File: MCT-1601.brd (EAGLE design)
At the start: 26.7 x 23.8 mm, 14 parts, among them J1 DUT, J2 Button, J3 D I/O, J5 A In, J6 Pwr, Q1 BC327

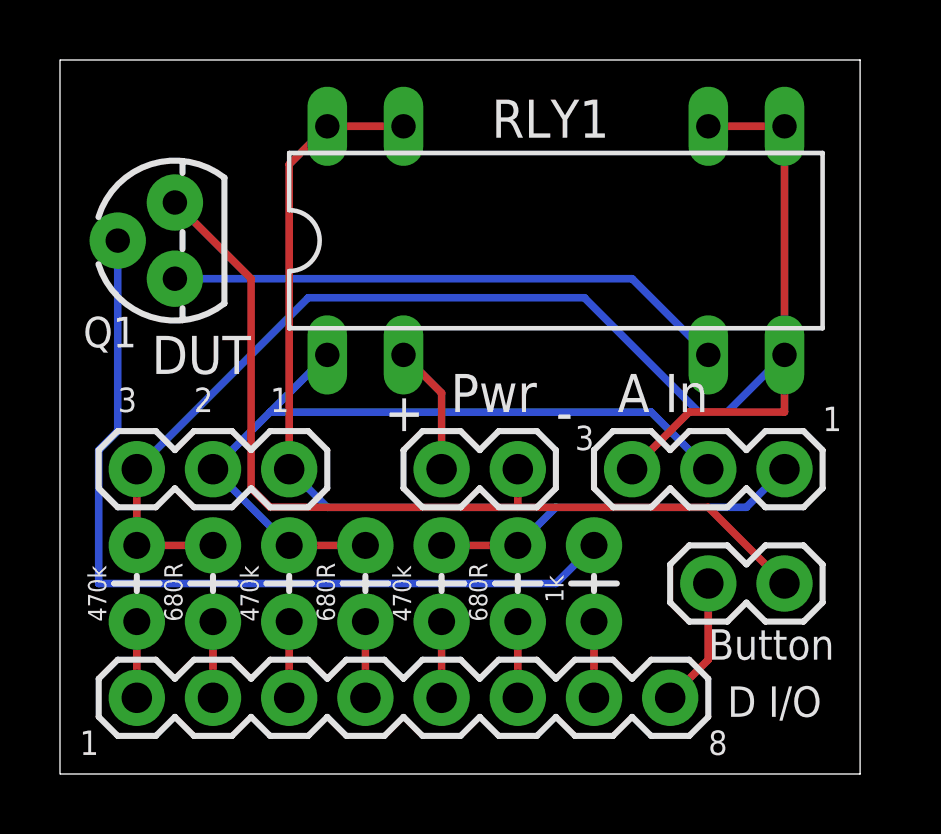
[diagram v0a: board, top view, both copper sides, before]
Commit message: Add files via upload
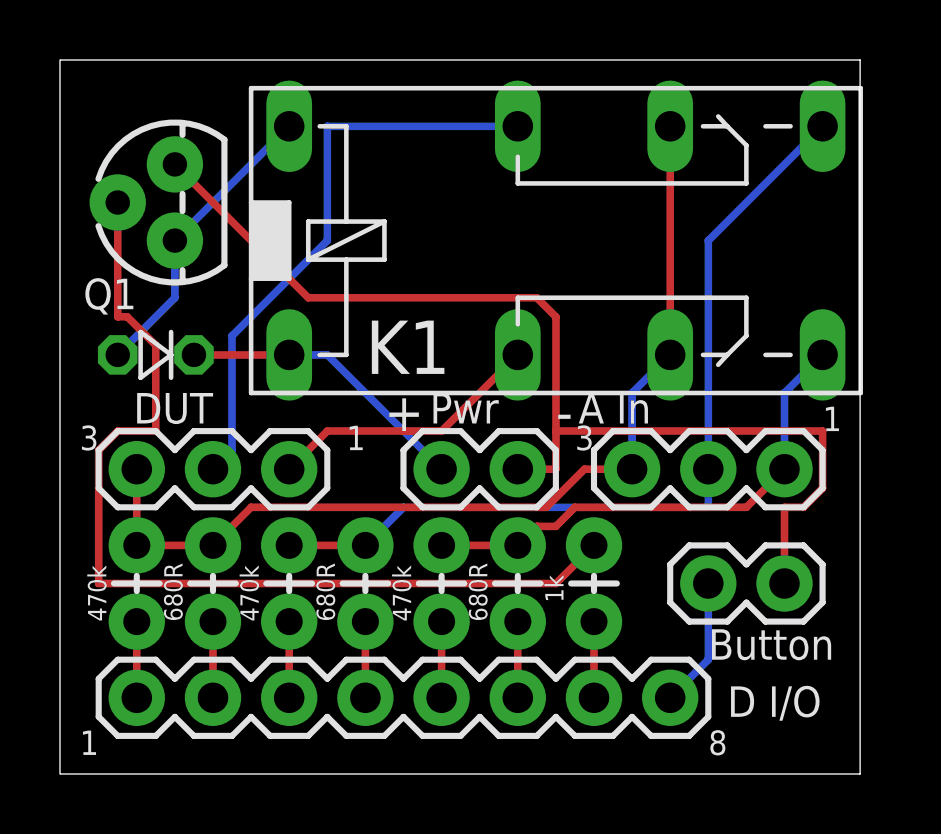
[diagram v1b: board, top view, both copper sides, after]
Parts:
- removed RLY1: W171-DIP-28, 00 Nik misc:DIL14-RELAY
- added D1: (no value), diode:D-2.5
- added K1: 351, relay:351
- moved Q1 1.27 mm to (3.81, 19.1)
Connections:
- new net N$1: J1.2, K1.P2
- new net N$4: J1.1, K1.P1
- net N$3: now also D1.A, K1.16; no longer RLY1.6
- net T1: now also K1.S1; no longer J1.1, RLY1.13, RLY1.14
- net T2: now also K1.S2; no longer J1.2, RLY1.1
- net T3: now also K1.O1, K1.O2; no longer RLY1.7, RLY1.8, RLY1.9
- net VCC: now also D1.C, K1.1; no longer RLY1.2
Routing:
- net T1: track 36.4 -> 16.8 mm
- net N$1: track 0.00 -> 19.4 mm
- net T3: track 49.3 -> 32.1 mm
- net N$4: track 0.00 -> 9.20 mm
- net N$3: track 18.8 -> 9.99 mm
- net VCC: track 4.34 -> 9.83 mm
- net GND: track 30.9 -> 36.0 mm
- net N$2: track 28.7 -> 32.0 mm
- net T2: track 26.9 -> 28.8 mm
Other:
- board text removed: "2"
